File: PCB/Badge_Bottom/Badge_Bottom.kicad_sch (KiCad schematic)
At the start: 26 parts, among them J1 Nylon Screw, J10 Debug, J2 Metal Screw, J3 Nylon Screw, J4 Metal Screw, J5 Nylon Screw, J6 Metal Screw, Q1 AO3400A, U2 CH32V305RBT6, Y1 8M

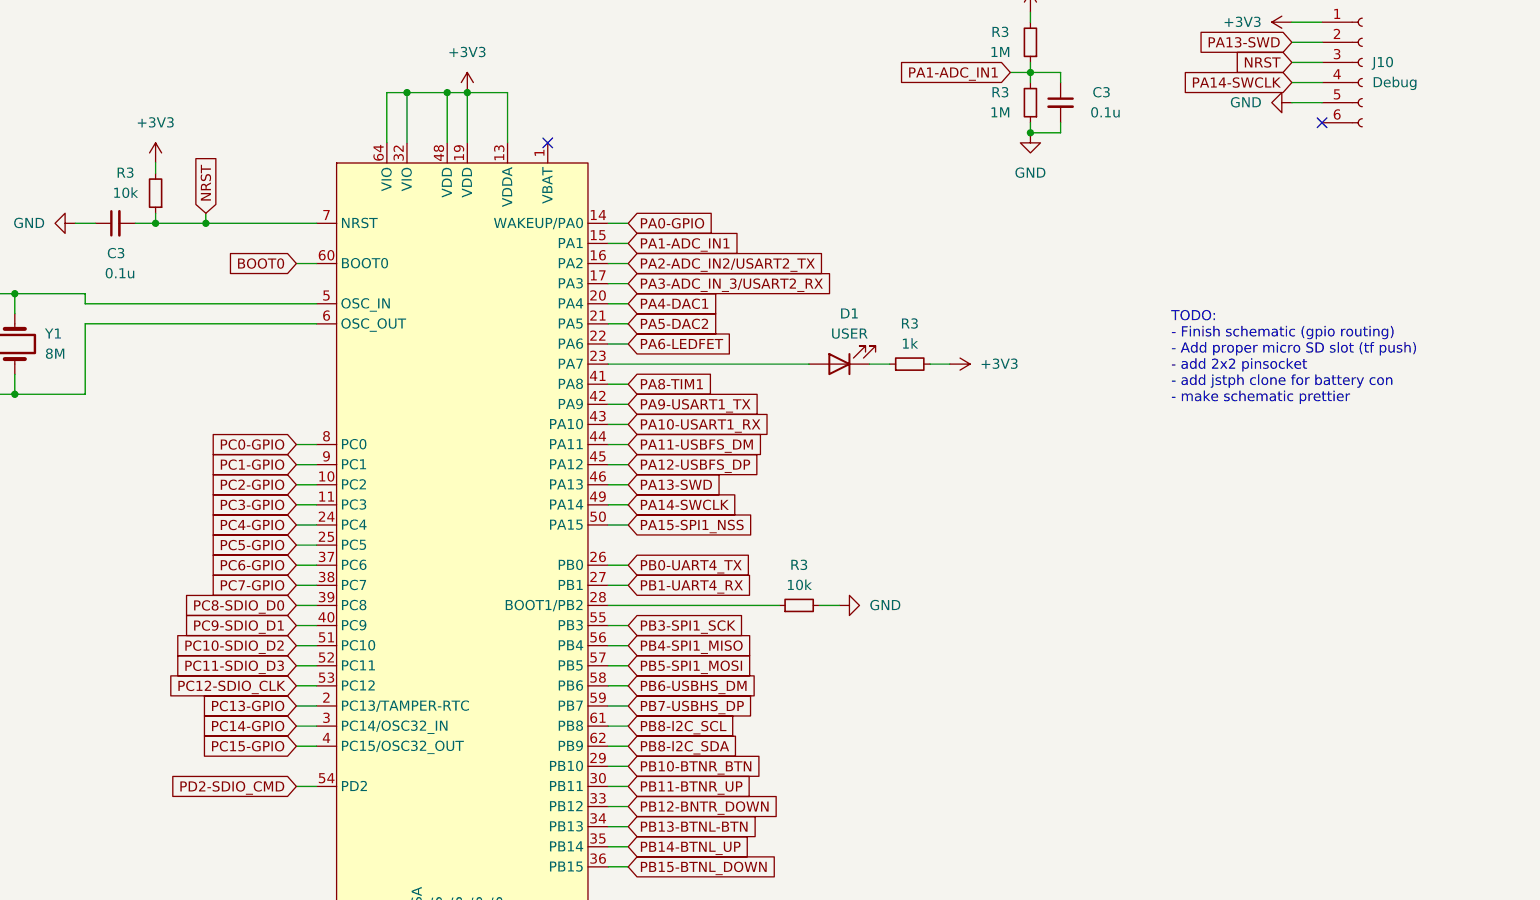
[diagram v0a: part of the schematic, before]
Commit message: finished schematic and added jlc parts
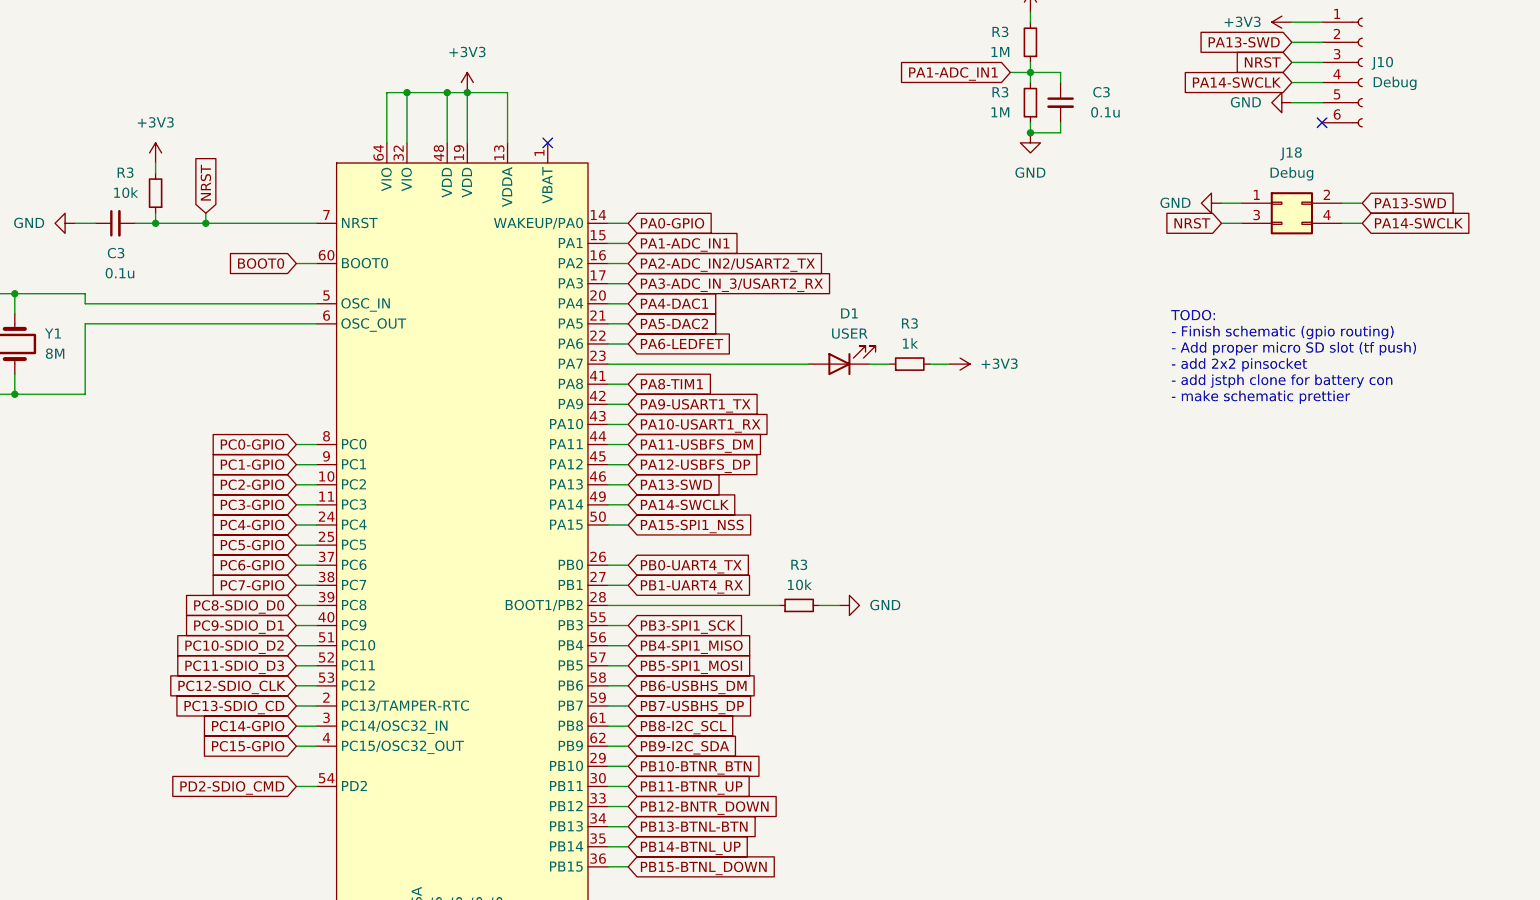
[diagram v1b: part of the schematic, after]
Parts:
- added J18: Debug, Connector_PinSocket_2.54mm:PinSocket_2x02_P2.54mm_Horizontal, symbol Connector_Generic:Conn_02x02_Odd_Even
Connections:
- net GND: now also J18.1 (Pin_1)
- net NRST: now also J18.3 (Pin_3)
- net PA13-SWD: now also J18.2 (Pin_2)
- net PA14-SWCLK: now also J18.4 (Pin_4)
- net PB8-I2C_SDA renamed PB9-I2C_SDA
- net PC13-GPIO renamed PC13-SDIO_CD
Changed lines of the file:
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@@
+    (stroke (width 0) (type default))
+  )
+  (wire (pts (xy 261.62 49.53) (xy 264.16 49.53))
     (stroke (width 0) (type default))
   )
@@
     (stroke (width 0) (type default))
   )
+  (wire (pts (xy 246.38 52.07) (xy 248.92 52.07))
+    (stroke (width 0) (type default))
+  )
   (wire (pts (xy 44.45 29.21) (xy 44.45 27.94))
     (stroke (width 0) (type default))
@@
     (stroke (width 0) (type default))
   )
+  (wire (pts (xy 246.38 49.53) (xy 248.92 49.53))
+    (stroke (width 0) (type default))
+  )
   (wire (pts (xy 21.59 20.32) (xy 24.13 20.32))
     (stroke (width 0) (type default))
@@
   )
   (wire (pts (xy 109.22 52.07) (xy 111.76 52.07))
+    (stroke (width 0) (type default))
+  )
+  (wire (pts (xy 261.62 52.07) (xy 264.16 52.07))
     (stroke (width 0) (type default))
   )
@@
     )
   )
-  (global_label "PB8-I2C_SDA" (shape input) (at 171.45 118.11 0) (fields_autoplaced)
+  (global_label "PB9-I2C_SDA" (shape input) (at 171.45 118.11 0) (fields_autoplaced)
     (effects (font (size 1.27 1.27)) (justify left))
     (property "Intersheetrefs" "${INTERSHEET_REFS}" (at 187.3771 118.11 0)
@@
     )
   )
+  (global_label "NRST" (shape input) (at 246.38 52.07 180) (fields_autoplaced)
+    (effects (font (size 1.27 1.27)) (justify right))
+    (property "Intersheetrefs" "${INTERSHEET_REFS}" (at 238.6172 52.07 0)
+      (effects (font (size 1.27 1.27)) (justify right) hide)
+    )
+  )
   (global_label "PC11-SDIO_D3" (shape input) (at 129.54 107.95 180) (fields_autoplaced)
     (effects (font (size 1.27 1.27)) (justify right))
@@
     )
   )
+  (global_label "PA14-SWCLK" (shape input) (at 264.16 52.07 0) (fields_autoplaced)
+    (effects (font (size 1.27 1.27)) (justify left))
+    (property "Intersheetrefs" "${INTERSHEET_REFS}" (at 279.7242 52.07 0)
+      (effects (font (size 1.27 1.27)) (justify left) hide)
+    )
+  )
   (global_label "PC0-GPIO" (shape input) (at 129.54 80.01 180) (fields_autoplaced)
     (effects (font (size 1.27 1.27)) (justify right))
@@
     )
   )
-  (global_label "PC13-GPIO" (shape input) (at 129.54 113.03 180) (fields_autoplaced)
+  (global_label "PC13-SDIO_CD" (shape input) (at 129.54 113.03 180) (fields_autoplaced)
     (effects (font (size 1.27 1.27)) (justify right))
     (property "Intersheetrefs" "${INTERSHEET_REFS}" (at 115.5481 113.03 0)
@@
     (property "Intersheetrefs" "${INTERSHEET_REFS}" (at 113.371 100.33 0)
       (effects (font (size 1.27 1.27)) (justify right) hide)
+    )
+  )
+  (global_label "PA13-SWD" (shape input) (at 264.16 49.53 0) (fields_autoplaced)
+    (effects (font (size 1.27 1.27)) (justify left))
+    (property "Intersheetrefs" "${INTERSHEET_REFS}" (at 277.4261 49.53 0)
+      (effects (font (size 1.27 1.27)) (justify left) hide)
     )
   )
@@
         (path "/9bea0129-61af-4534-9a88-a88b63234707/0f55777b-99bc-476f-91c2-8f0549bc7bba"
           (reference "#PWR014") (unit 1)
+        )
+      )
+    )
+  )
+  (symbol (lib_id "Connector_Generic:Conn_02x02_Odd_Even") (at 254 49.53 0) (unit 1)
+    (in_bom yes) (on_board yes) (dnp no) (fields_autoplaced)
+    (property "Reference" "J18" (at 255.27 43.18 0)
+      (effects (font (size 1.27 1.27)))
+    )
+    (property "Value" "Debug" (at 255.27 45.72 0)
+      (effects (font (size 1.27 1.27)))
+    )
+    (property "Footprint" "Connector_PinSocket_2.54mm:PinSocket_2x02_P2.54mm_Horizontal" (at 254 49.53 0)
+      (effects (font (size 1.27 1.27)) hide)
+    )
+    (property "Datasheet" "~" (at 254 49.53 0)
+      (effects (font (size 1.27 1.27)) hide)
+    )
+    (pin "1")
+    (pin "2")
+    (pin "3")
+    (pin "4")
+    (instances
+      (project "Badge_Bottom"
+        (path "/9bea0129-61af-4534-9a88-a88b63234707/8d25bc71-ccea-4834-b12f-ddce477db9bd"
+          (reference "J18") (unit 1)
+        )
+        (path "/9bea0129-61af-4534-9a88-a88b63234707"
+          (reference "J20") (unit 1)
         )
       )
@@
         )
       )
+    )
+  )
+  (symbol (lib_id "power:GND") (at 246.38 49.53 270) (unit 1)
+    (in_bom yes) (on_board yes) (dnp no) (fields_autoplaced)
+    (property "Reference" "#PWR055" (at 240.03 49.53 0)
+      (effects (font (size 1.27 1.27)) hide)
+    )
+    (property "Value" "GND" (at 242.57 49.53 90)
+      (effects (font (size 1.27 1.27)) (justify right))
+    )
+    (property "Footprint" "" (at 246.38 49.53 0)
+      (effects (font (size 1.27 1.27)) hide)
+    )
+    (property "Datasheet" "" (at 246.38 49.53 0)
+      (effects (font (size 1.27 1.27)) hide)
+    )
+    (pin "1")
+    (instances
+      (project "Badge_Bottom"
+        (path "/9bea0129-61af-4534-9a88-a88b63234707"
+          (reference "#PWR055") (unit 1)
+        )
+      )

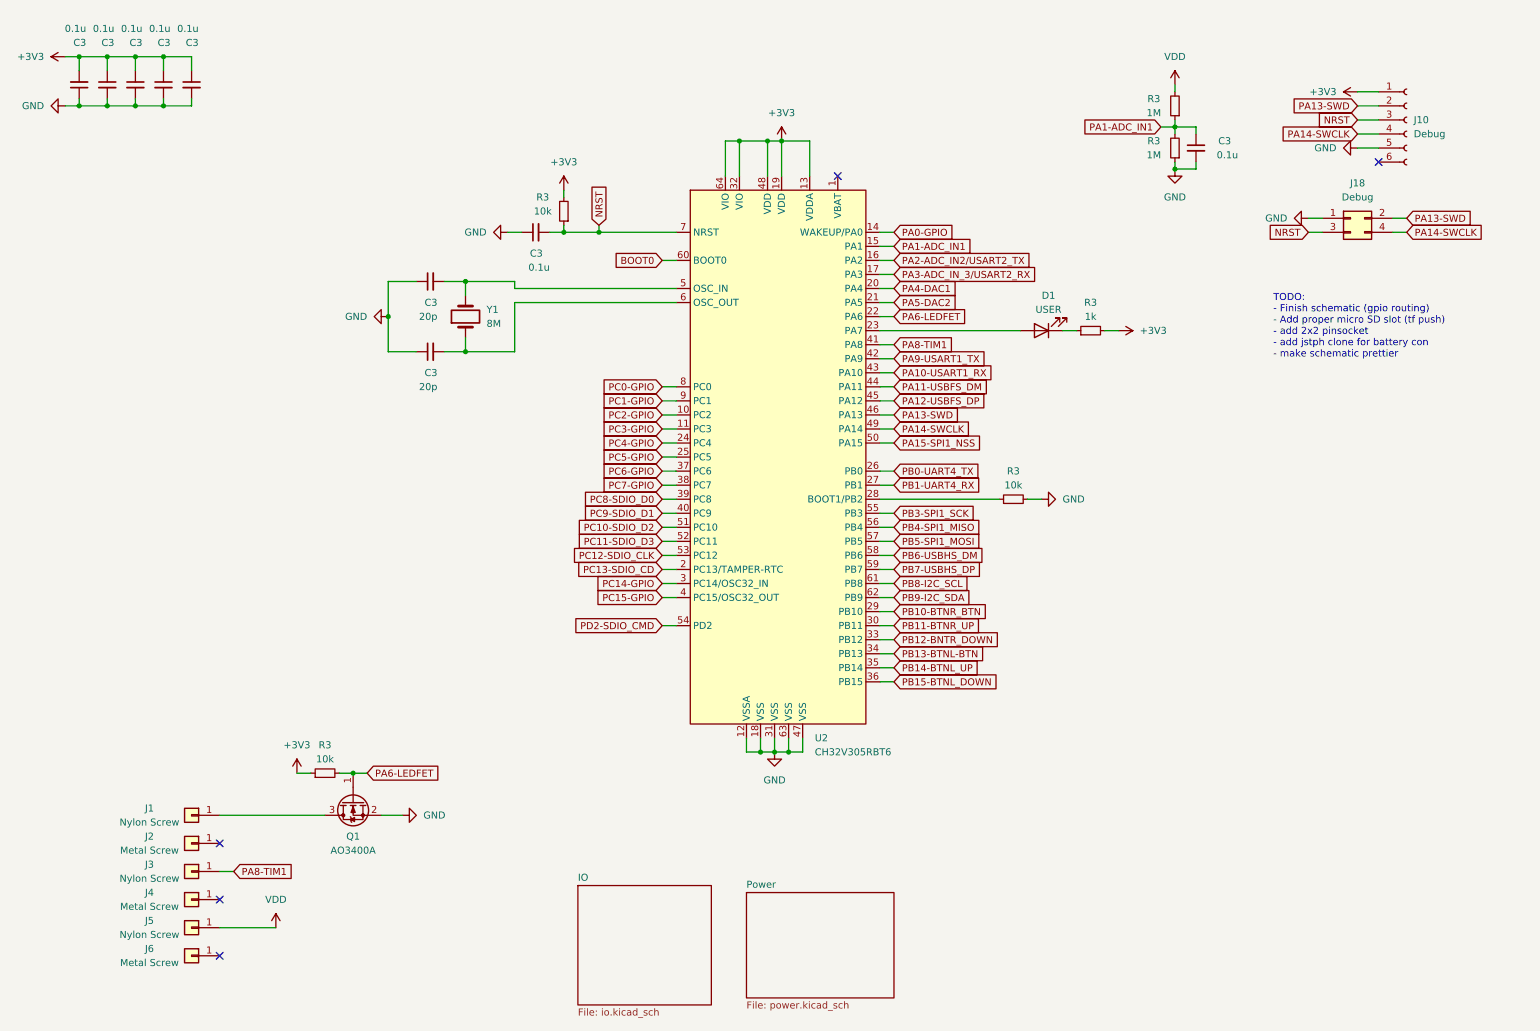
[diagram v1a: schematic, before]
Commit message: finised pcb layout
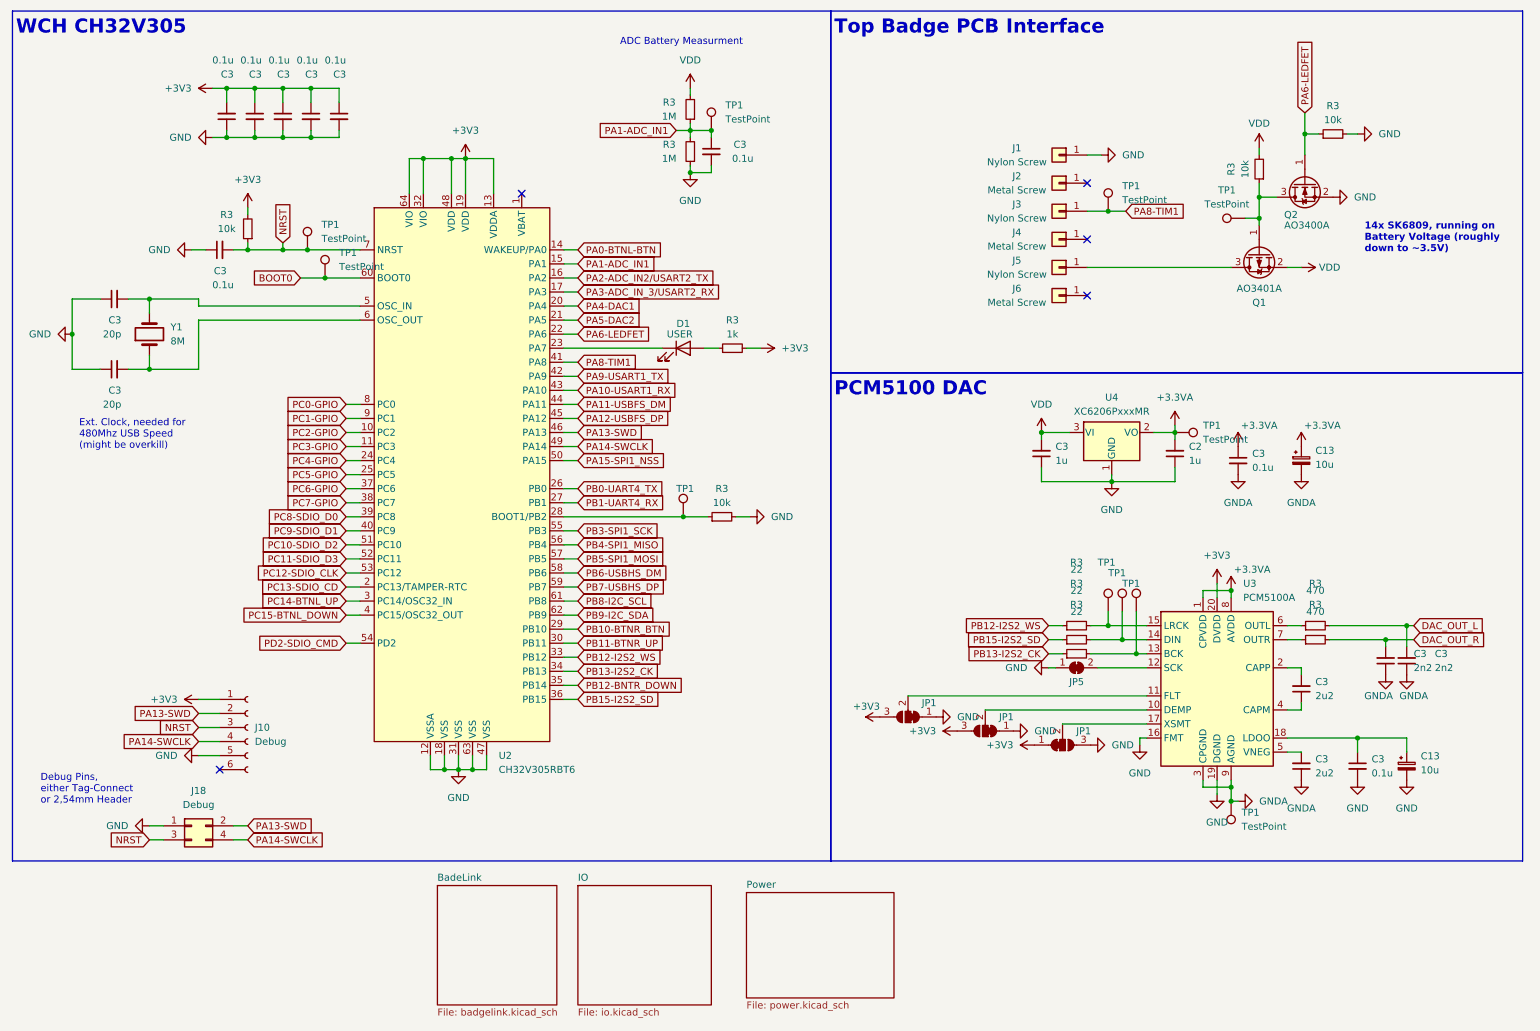
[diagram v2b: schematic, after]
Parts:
- removed Q1: AO3400A, Package_TO_SOT_SMD:SOT-23, symbol Transistor_FET:AO3400A
- added C13 (x2): 10u, Capacitor_Tantalum_SMD:CP_EIA-3216-18_Kemet-A, symbol Device:C_Polarized_Small
- added C2, C3: 1u, Capacitor_SMD:C_0603_1608Metric, symbol Device:C_Small
- added C3 (x2): 2u2, Capacitor_SMD:C_0603_1608Metric, symbol Device:C_Small
- added C3 (x2): 2n2, Capacitor_SMD:C_0603_1608Metric, symbol Device:C_Small
- added C3 (x2): 0.1u, Capacitor_SMD:C_0603_1608Metric, symbol Device:C_Small
- added JP1 (x3): SolderJumper_3_Bridged12, Jumper:SolderJumper-3_P1.3mm_Bridged12_RoundedPad1.0x1.5mm, symbol Jumper:SolderJumper_3_Bridged12
- added JP5: SolderJumper_2_Bridged, Jumper:SolderJumper-2_P1.3mm_Bridged_RoundedPad1.0x1.5mm, symbol Jumper:SolderJumper_2_Bridged
- added Q1: AO3401A, Package_TO_SOT_SMD:SOT-23, symbol Transistor_FET:AO3401A
- added Q2: AO3400A, Package_TO_SOT_SMD:SOT-23, symbol Transistor_FET:AO3400A
- added R3 (x2): 470, Resistor_SMD:R_0603_1608Metric, symbol Device:R_Small
- added R3 (x3): 22, Resistor_SMD:R_0603_1608Metric, symbol Device:R_Small
- added R3: 10k, Resistor_SMD:R_0603_1608Metric, symbol Device:R_Small
- added TP1 (x11): TestPoint, TestPoint:TestPoint_Pad_D1.0mm, symbol Connector:TestPoint
- added U3: PCM5100A, Package_SO:TSSOP-20_4.4x6.5mm_P0.65mm, symbol Audio:PCM5100A
- added U4: XC6206PxxxMR, Package_TO_SOT_SMD:SOT-23-3, symbol Regulator_Linear:XC6206PxxxMR
- J18: footprint Connector_PinSocket_2.54mm:PinSocket_2x02_P2.54mm_Horizontal -> 2x02_pinsocket_254:HDR-TH_4P-P2.54-H-F-R2-C2-W8.5
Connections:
- net PB14-BTNL_UP is gone; now on net PB12-BNTR_DOWN: U2.35 (PB14)
- net +3V3: now also JP1.1 (A), JP1.3 (B), JP1.3 (B), U3.20 (DVDD); no longer R3.1
- net BOOT0: now also TP1.1
- net GND: now also J1.1 (Pin_1), C13.2, C2.1, C3.1, C3.2, JP1.1 (A), JP1.1 (A), JP1.3 (B), JP5.1 (A), Q2.2 (S), R3.2, U3.16 (FMT), U3.19 (DGND), U4.1 (GND)
- net NRST: now also TP1.1
- net PA1-ADC_IN1: now also TP1.1
- net PA6-LEDFET: now also Q2.1 (G), R3.1; no longer R3.2
- net PA8-TIM1: now also TP1.1
- net PB12-BNTR_DOWN: no longer U2.33 (PB12)
- net VDD: now also R3.2, C3.2, Q1.2 (S), U4.3 (VI); no longer J5.1 (Pin_1)
- net at R3.1, U2.28 (BOOT1/PB2): now also TP1.1
- net at U2.23 (PA7): now also D1.1 (K); no longer D1.2 (A)
- net at R3.1: now also D1.2 (A); no longer D1.1 (K)
- net PA0-GPIO renamed PA0-BTNL-BTN
- net PB13-BTNL-BTN renamed PB13-I2S2_CK
- net PB13-I2S2_CK: now also R3.1
- net PB15-BTNL_DOWN renamed PB15-I2S2_SD
- net PB15-I2S2_SD: now also R3.1
- net PC14-GPIO renamed PC14-BTNL_UP
- net PC15-GPIO renamed PC15-BTNL_DOWN
- new net: C3.2, U3.5 (VNEG)
- new net: R3.1, U3.6 (OUTL)
- new net: R3.2, TP1.1, U3.14 (DIN)
- new net: R3.2, TP1.1, U3.13 (BCK)
- new net: JP1.2 (C), U3.11 (FLT)
- new net: Q1.1 (G), Q2.3 (D), R3.1, TP1.1
- new net: J5.1 (Pin_1), Q1.3 (D)
- new net: R3.1, U3.7 (OUTR)
- new net: R3.2, TP1.1, U3.15 (LRCK)
- new net: JP1.2 (C), U3.17 (XSMT)
- new net: C3.1, U3.4 (CAPM)
- new net: C3.2, U3.2 (CAPP)
- new net: C13.1, C3.1, U3.18 (LDOO)
- new net: JP1.2 (C), U3.10 (DEMP)
- new net: JP5.2 (B), U3.12 (SCK)
- new net +3.3VA: C13.1, C2.2, C3.1, TP1.1, U3.1 (CPVDD), U3.8 (AVDD), U4.2 (VO)
- new net DAC_OUT_L: C3.2, R3.2
- new net DAC_OUT_R: C3.2, R3.2
- new net GNDA: C13.2, C3.1, C3.1, C3.1, C3.2, TP1.1, U3.3 (CPGND), U3.9 (AGND)
- new net PB12-I2S2_WS: R3.1, U2.33 (PB12)
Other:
- added sheet BadeLink (badgelink.kicad_sch)
- note added: "14x SK6809, running on Battery Voltage (roughly down to ~3.5V)"
- note added: "ADC Battery Measurment"
- note added: "Debug Pins, either Tag-Connect or 2,54mm Header"
- note added: "Ext. Clock, needed for 480Mhz USB Speed (might be overkill)"
- note added: "PCM5100 DAC"
- note added: "Top Badge PCB Interface"
- note added: "WCH CH32V305"
- note removed: "TODO: - Finish schematic (gpio routing) - Add proper micro SD slot (tf push) - add 2x2 pinsocket - add jstph clone for battery con - make schematic prettier"
- moved on the sheet: C3, D1, J1, J10, J18, J2, J3, J4, J5, J6, R3, U2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

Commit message: Added docs and readme, ordered PCBs at JLC
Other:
- company: (none) -> Unterland
- title: (none) -> Unterland Badge Bottom
